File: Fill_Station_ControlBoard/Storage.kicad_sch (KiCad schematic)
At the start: 15 parts, among them J5 Micro_SD_Card_Det1

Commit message: Fait des trucs (commencer arrangement de pièces sur PCB
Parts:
- J5: footprint (none) -> Connector_Card:microSD_HC_Hirose_DM3AT-SF-PEJM5
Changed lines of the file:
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@@
 			)
 		)
-		(property "Footprint" ""
+		(property "Footprint" "Connector_Card:microSD_HC_Hirose_DM3AT-SF-PEJM5"
 			(at 231.14 72.39 0)
 			(effects

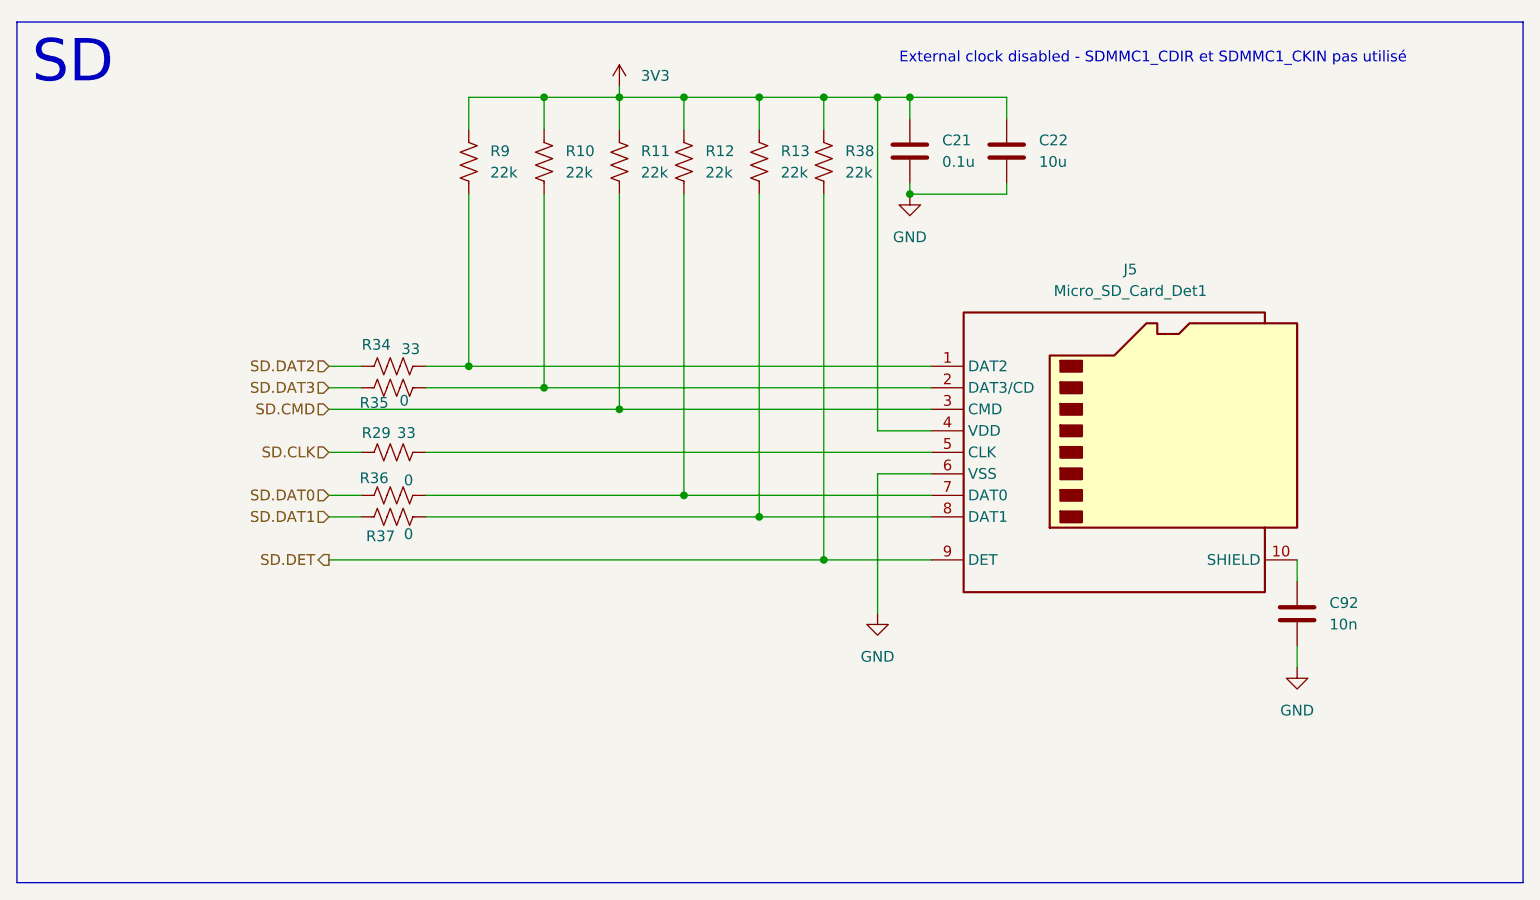
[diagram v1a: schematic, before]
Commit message: arthur
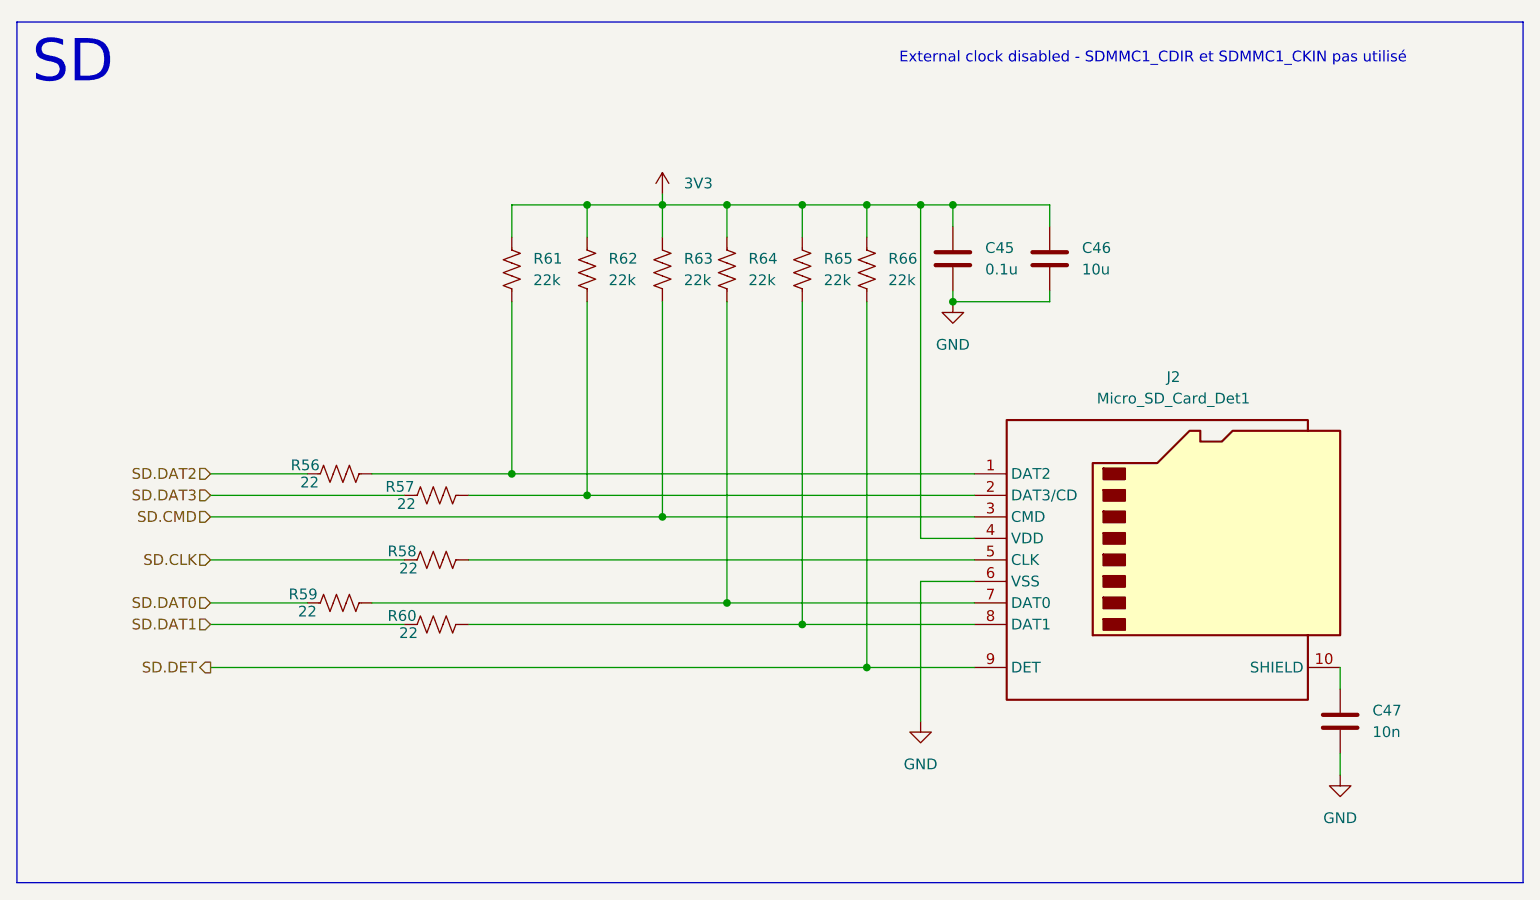
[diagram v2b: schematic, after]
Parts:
- removed C21: 0.1u, Capacitor_SMD:C_0603_1608Metric, symbol Device:C
- removed C22: 10u, Capacitor_SMD:C_0603_1608Metric, symbol Device:C
- removed C92: 10n, Capacitor_SMD:C_0603_1608Metric, symbol Device:C
- removed J5: Micro_SD_Card_Det1, Connector_Card:microSD_HC_Hirose_DM3AT-SF-PEJM5, symbol Connector:Micro_SD_Card_Det1
- removed R10, R11, R12, R13, R38, R9: 22k, Resistor_SMD:R_0603_1608Metric_Pad0.98x0.95mm_HandSolder, symbol Device:R_US
- removed R29, R34: 33, Resistor_SMD:R_0603_1608Metric_Pad0.98x0.95mm_HandSolder, symbol Device:R_US
- removed R35, R36, R37: 0, Resistor_SMD:R_0603_1608Metric_Pad0.98x0.95mm_HandSolder, symbol Device:R_US
- added C45: 0.1u, symbol Device:C
- added C46: 10u, symbol Device:C
- added C47: 10n, symbol Device:C
- added J2: Micro_SD_Card_Det1, symbol Connector:Micro_SD_Card_Det1
- added R56, R57, R58, R59, R60: 22, symbol Device:R_US
- added R61, R62, R63, R64, R65, R66: 22k, symbol Device:R_US
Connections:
- net 3V3: now also C45.1, C46.1, J2.4 (VDD), R61.1, R62.1, R63.1, R64.1, R65.1, R66.1
- net GND: now also C45.2, C46.2, C47.2, J2.6 (VSS)
- net SD.CLK: now also R58.1
- net SD.CMD: now also J2.3 (CMD), R63.2
- net SD.DAT0: now also R59.1
- net SD.DAT1: now also R60.1
- net SD.DAT2: now also R56.1
- net SD.DAT3: now also R57.1
- net SD.DET: now also J2.9 (DET), R66.2
- new net: J2.5 (CLK), R58.2
- new net: C47.1, J2.10 (SHIELD)
- new net: J2.7 (DAT0), R59.2, R64.2
- new net: J2.8 (DAT1), R60.2, R65.2
- new net: J2.2 (DAT3/CD), R57.2, R62.2
- new net: J2.1 (DAT2), R56.2, R61.2
